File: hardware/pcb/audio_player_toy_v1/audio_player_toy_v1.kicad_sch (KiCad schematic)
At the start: 21 parts, among them J1 Conn_02x05_Odd_Even, U1 BH-AAA-B5AA005, U2 ISD2360YYI

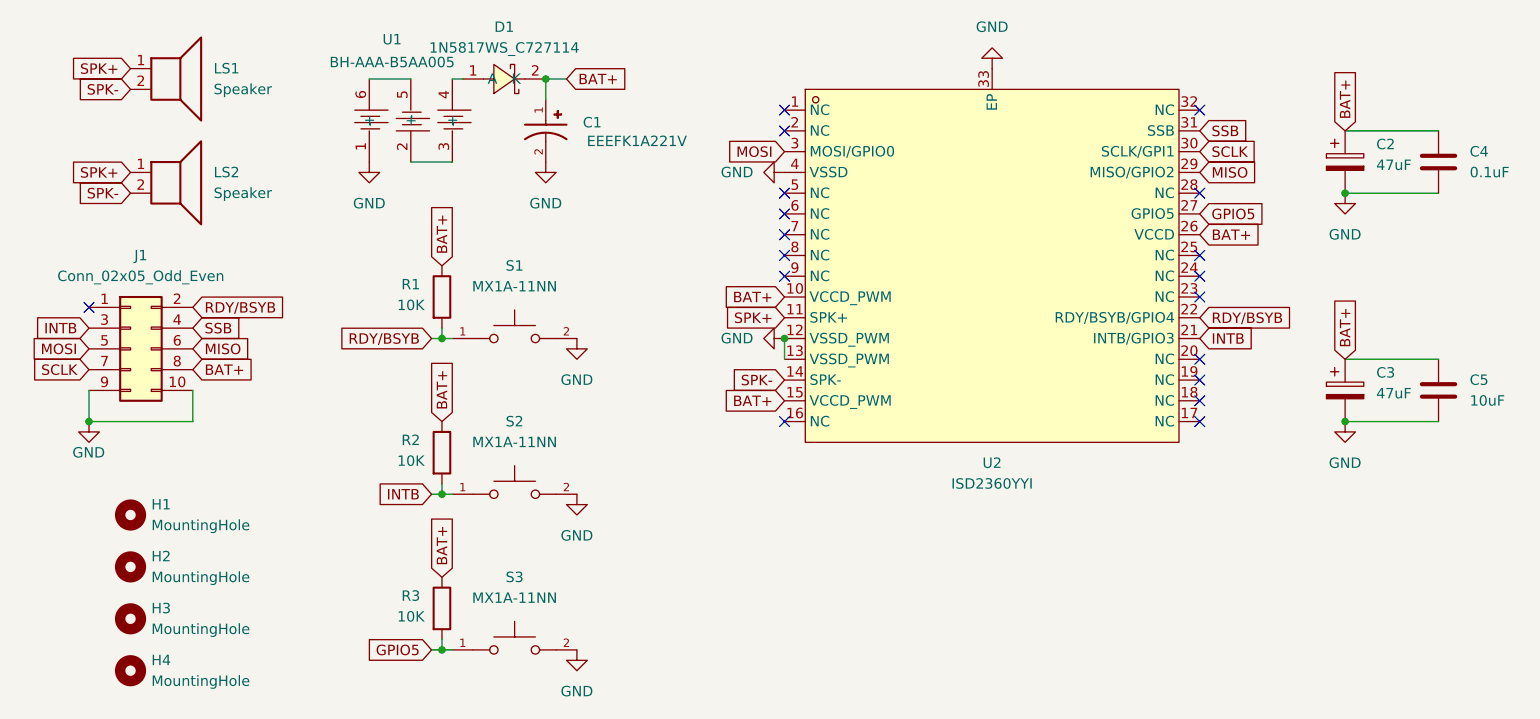
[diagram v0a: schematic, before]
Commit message: feat: complete sch and pcb of v1
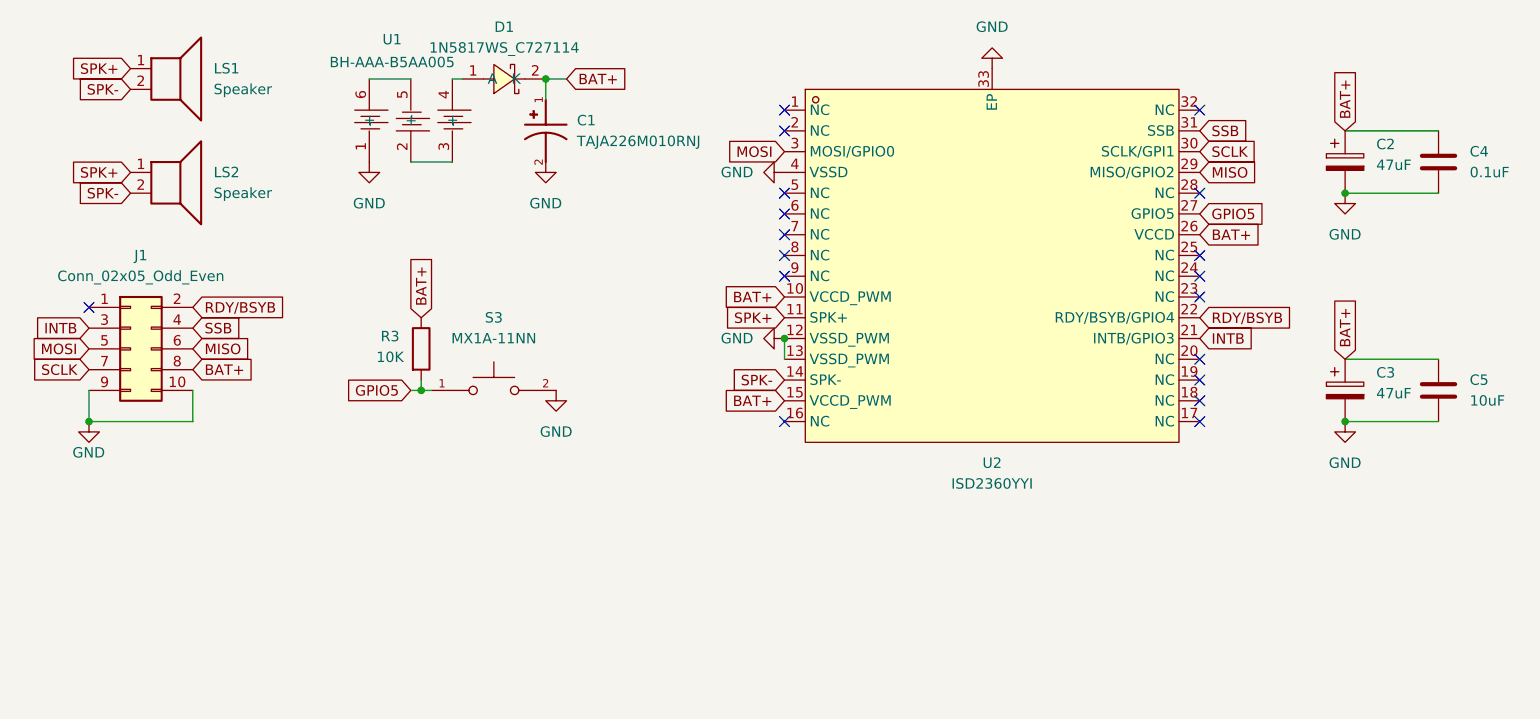
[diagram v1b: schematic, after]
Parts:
- removed C1: EEEFK1A221V, .pretty:CAP_EEEFK1A221V, symbol EEEFK1A221V:EEEFK1A221V
- removed H1, H2, H3, H4: MountingHole, MountingHole:MountingHole_3.2mm_M3, symbol Mechanical:MountingHole
- removed R1, R2: 10K, Resistor_SMD:R_0603_1608Metric, symbol Device:R
- removed S1, S2: MX1A-11NN, .pretty:SW_MX1A-11NN, symbol MX1A-11NN:MX1A-11NN
- added C1: TAJA226M010RNJ, .pretty:CAPMP3216X180N, symbol TAJA226M010RNJ:TAJA226M010RNJ
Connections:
- net BAT+: now also C1.1
- net GND: now also C1.2
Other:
- moved on the sheet: R3, S3
